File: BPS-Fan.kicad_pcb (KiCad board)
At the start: 2 copper layers, 57.3 x 82.1 mm, 37 parts, among them J1 LDRBRDConn, J10 FAN9, J11 FAN10, J12 FAN11, J13 FAN12, J2 FAN1, J3 FAN2, J4 FAN3, J5 FAN4, J6 FAN5, J7 FAN6, J8 FAN7, J9 FAN8, Q1 BUK9M23-80E, Q2 BUK9M23-80E, Q3 BUK9M23-80E, Q4 BUK9M23-80E

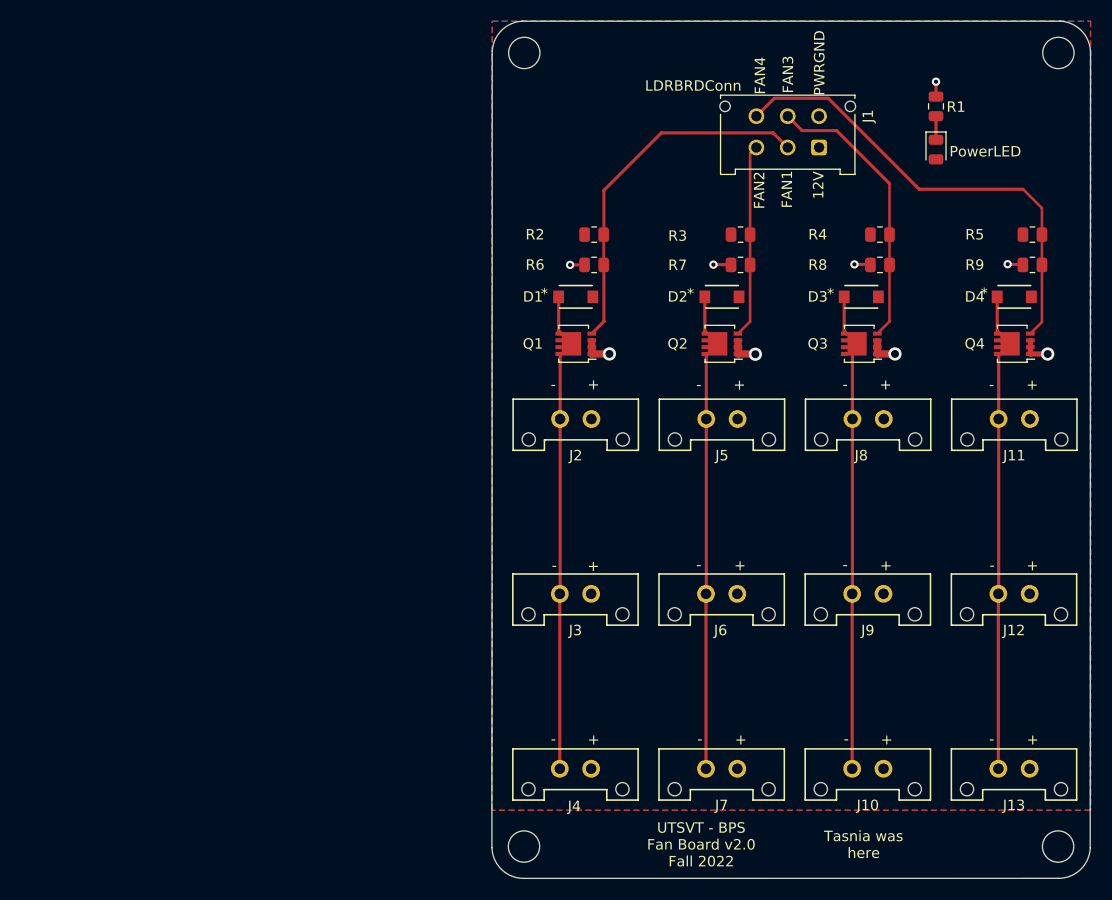
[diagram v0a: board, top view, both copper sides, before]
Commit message: fan go brrr
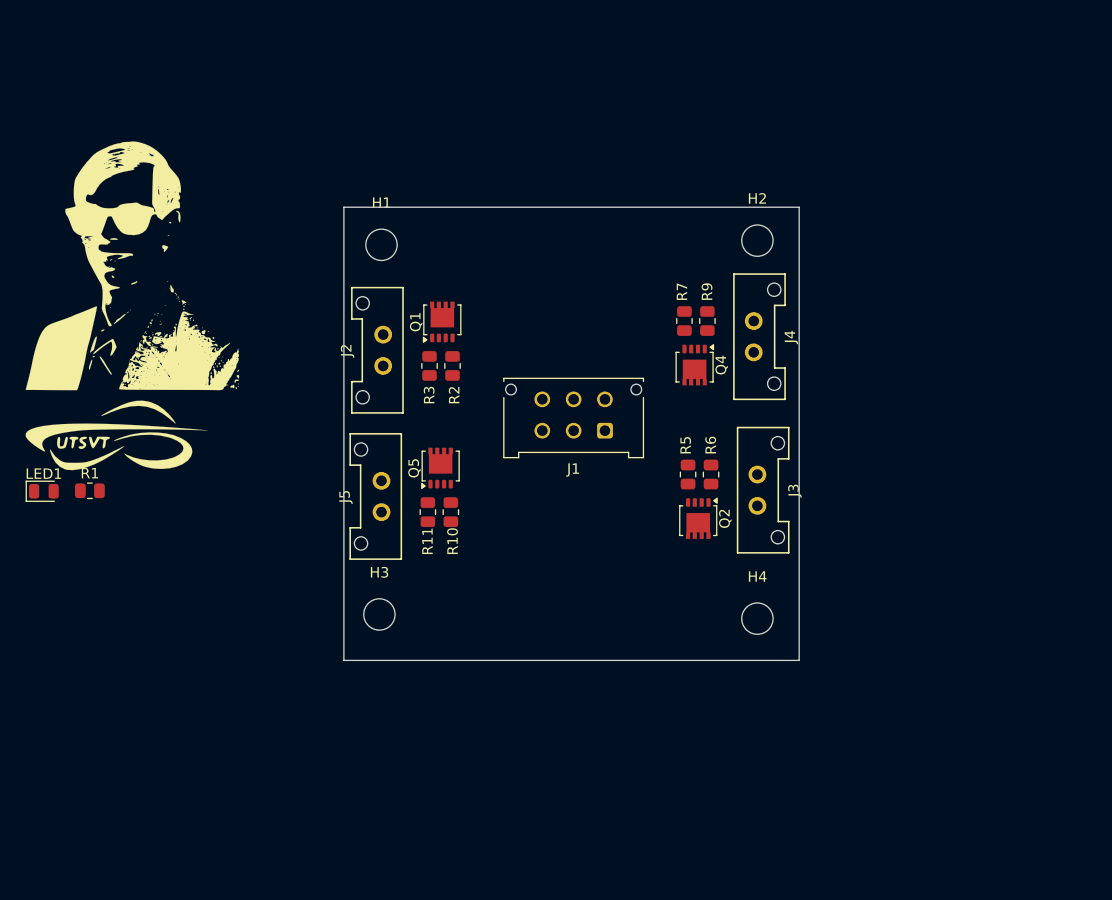
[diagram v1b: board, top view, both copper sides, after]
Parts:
- removed D1, D2, D3, D4: V2F22HM, UTSVT_Passive:V2F22HM
- removed J10: FAN9, UTSVT_Connectors:Molex_MicroFit3.0_1x2xP3.00mm_PolarizingPeg_Vertical
- removed J11: FAN10, UTSVT_Connectors:Molex_MicroFit3.0_1x2xP3.00mm_PolarizingPeg_Vertical
- removed J12: FAN11, UTSVT_Connectors:Molex_MicroFit3.0_1x2xP3.00mm_PolarizingPeg_Vertical
- removed J13: FAN12, UTSVT_Connectors:Molex_MicroFit3.0_1x2xP3.00mm_PolarizingPeg_Vertical
- removed J6: FAN5, UTSVT_Connectors:Molex_MicroFit3.0_1x2xP3.00mm_PolarizingPeg_Vertical
- removed J7: FAN6, UTSVT_Connectors:Molex_MicroFit3.0_1x2xP3.00mm_PolarizingPeg_Vertical
- removed J8: FAN7, UTSVT_Connectors:Molex_MicroFit3.0_1x2xP3.00mm_PolarizingPeg_Vertical
- removed J9: FAN8, UTSVT_Connectors:Molex_MicroFit3.0_1x2xP3.00mm_PolarizingPeg_Vertical
- removed PowerLED: STATUS, LED_SMD:LED_0805_2012Metric
- removed Q3: BUK9M23-80E, Package_TO_SOT_SMD:LFPAK33
- removed R4, R8: 100k, Resistor_SMD:R_0805_2012Metric
- added LED1: STATUS, LED_SMD:LED_0805_2012Metric, F.Cu at (85.6, 85.7)
- added Q5: BUK9M23-80E, Package_TO_SOT_SMD:LFPAK33, F.Cu at (123.6, 83.5)
- added R10: 100k, Resistor_SMD:R_0805_2012Metric, F.Cu at (124.5, 87.7)
- added R11: 100k, Resistor_SMD:R_0805_2012Metric, F.Cu at (122.3, 87.7)
- J2: value FAN1 -> FAN7
- J3: value FAN2 -> FAN7
- J4: value FAN3 -> FAN7
- J5: value FAN4 -> FAN7
- LOGO1, LOGO2: moved to F.Cu
- moved R1 89.0 mm to (90.0, 85.7), turned to 0 degrees
- moved H3 84.4 mm to (117.7, 97.5)
- moved LOGO2 68.4 mm to (92.3, 80.5), turned to 0 degrees
- moved H2 64.8 mm to (153.9, 61.7)
- moved LOGO1 48.7 mm to (93.2, 63.8), turned to 0 degrees
- moved J4 45.6 mm to (153.5, 69.4), turned to -90 degrees
- moved R5 40.2 mm to (147.3, 84.1), turned to -90 degrees
- moved J5 35.3 mm to (117.9, 87.7), turned to 90 degrees
- moved J1 34.0 mm to (139.3, 79.9)
- moved R3 32.3 mm to (122.5, 73.7), turned to -90 degrees
- moved R9 31.6 mm to (149.1, 69.4), turned to 90 degrees
- moved H4 31.2 mm to (153.9, 97.9)
- moved Q4 30.7 mm to (147.9, 73.6), turned to -90 degrees
- moved R6 23.0 mm to (149.5, 84.1), turned to 90 degrees
- moved H1 22.9 mm to (117.9, 62.1)
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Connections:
- J2 pad 2: Net-(D1-Pad2) -> Net-(D1-A)
- J3 pad 2: Net-(D1-Pad2) -> Net-(D2-A)
- J4 pad 2: Net-(D1-Pad2) -> Net-(D4-A)
- J5 pad 2: Net-(D2-Pad2) -> Net-(D5-A)
- Q1 pad 5: Net-(D1-Pad2) -> Net-(D1-A)
- Q2 pad 5: Net-(D2-Pad2) -> Net-(D2-A)
- Q4 pad 4: /FAN4_BPS -> /FAN3_BPS
- Q4 pad 5: Net-(D4-Pad2) -> Net-(D4-A)
- R3 pad 1: +12V -> /FAN1_BPS
- R3 pad 2: /FAN2_BPS -> GNDPWR
- R5 pad 2: /FAN4_BPS -> /FAN2_BPS
- R6 pad 1: /FAN1_BPS -> /FAN2_BPS
- R7 pad 1: /FAN2_BPS -> +12V
- R7 pad 2: GNDPWR -> /FAN3_BPS
- R9 pad 1: /FAN4_BPS -> /FAN3_BPS
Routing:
- net Net-(D4-Pad2): track 46.2 -> 0.00 mm
- net Net-(D2-Pad2): track 46.2 -> 0.00 mm
- net Net-(D1-Pad2): track 46.2 -> 0.00 mm
- net Net-(D3-Pad2): track 45.9 -> 0.00 mm
- net /FAN4_BPS: track 44.9 -> 0.00 mm
- net /FAN1_BPS: track 34.6 -> 0.00 mm
- net /FAN3_BPS: track 27.3 -> 0.00 mm
- net GNDPWR: track 19.1 -> 0.00 mm, vias 9 -> 0
- net /FAN2_BPS: track 18.6 -> 0.00 mm
- net Net-(LED1-K): track 2.16 -> 0.00 mm
- removed copper zone on F.Cu, net +12V
- removed copper zone on B.Cu, net GNDPWR
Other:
- board size 57.3 x 82.1 mm -> 43.6 x 43.4 mm
- board text removed: "+"
- board text removed: "-"
- board text removed: "12V"
- board text removed: "FAN1"
- board text removed: "FAN2"
- board text removed: "FAN3"
- board text removed: "FAN4"
- board text removed: "LDRBRDConn"
- board text removed: "PWRGND"
- board text removed: "Tasnia was here"
- board text removed: "UTSVT - BPS Fan Board v2.0 Fall 2022"
